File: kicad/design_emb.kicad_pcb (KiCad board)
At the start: 2 copper layers, 79.9 x 98.8 mm, 116 parts, among them J1 Conn_01x04, J2 Barrel_Jack, J3 USB_A, J4 Conn_01x03, J5 Conn_02x11_Counter_Clockwise, J6 Conn_02x10_Counter_Clockwise, J7 Screw_Terminal_01x02, J8 Screw_Terminal_01x02, K1 SANYOU_SRD_Form_C, K2 SANYOU_SRD_Form_C, Q1 MMBT3904, Q2 MMBT3904, SW1 SW_Push, SW3 SW_Push, U1 SRX.X.TCT, U10 S25FL116KOXNFIQ-11, U2 SRX.X.TCT, U3 STM32F446ZETx, U4 ICE40HX1K, U5 TLV1117LV33DCYR, U6 TLV1117LV33DCYR, U7 TLV1117LV12DCYR, U8 OMEGA2, U9 RCLAMP0502B

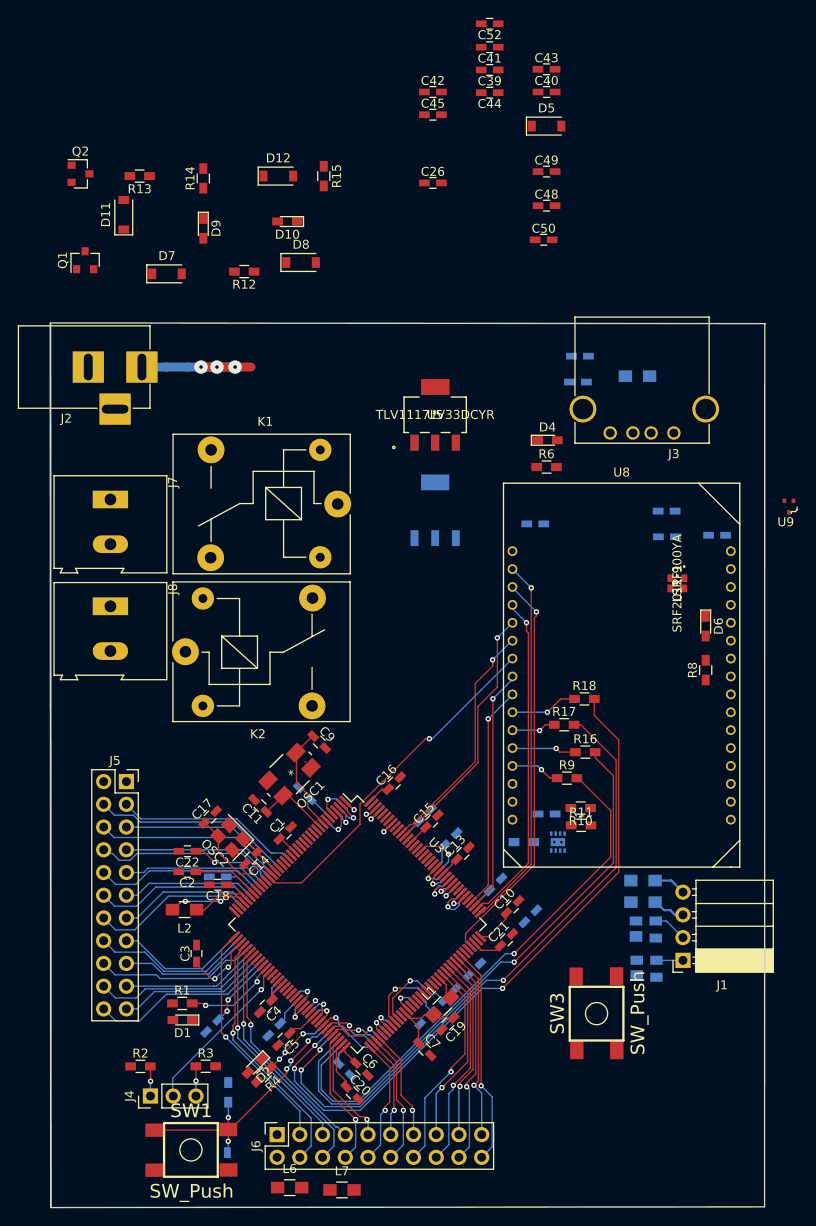
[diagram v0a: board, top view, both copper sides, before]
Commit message: ruteo
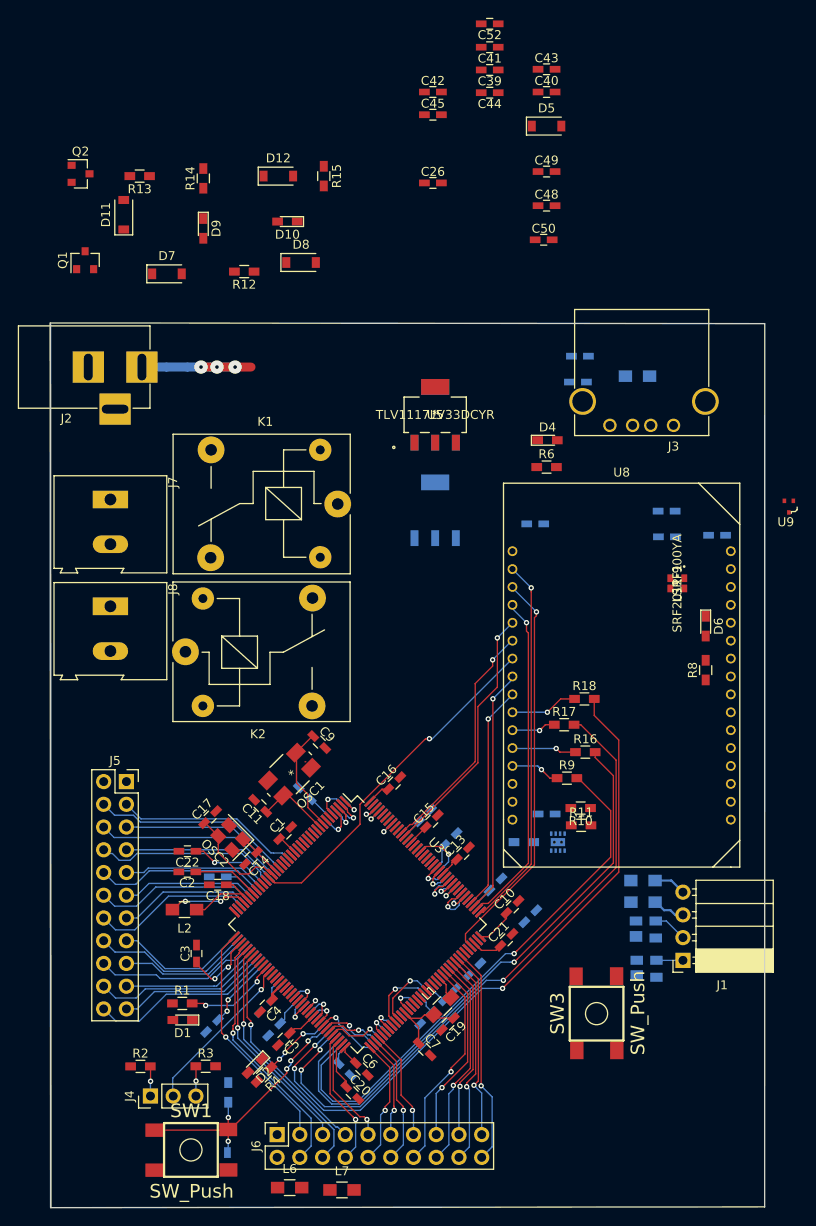
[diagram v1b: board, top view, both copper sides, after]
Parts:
- moved J3 0.85 mm to (148.8, 94.4)
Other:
- board size 79.9 x 98.8 mm -> 79.8 x 98.9 mm
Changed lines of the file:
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@@
   )
   (module Connectors:USB_A (layer F.Cu)
-    (at 148.844 95.25 180)
+    (at 148.8059 94.3991 180)
     (descr "USB A connector")
     (tags "USB USB_A")
@@
     )
   )
-  (gr_line (start 159.0802 83.0326) (end 79.1718 82.9564) (layer Edge.Cuts) (width 0.15))
-  (gr_line (start 158.9786 181.6989) (end 159.004 83.058) (layer Edge.Cuts) (width 0.15))
-  (gr_line (start 79.2353 181.7878) (end 79.1845 82.9818) (layer Edge.Cuts) (width 0.2))
+  (gr_line (start 158.9913 83.0326) (end 79.1718 82.9564) (layer Edge.Cuts) (width 0.15))
+  (gr_line (start 158.9913 181.7243) (end 159.004 83.058) (layer Edge.Cuts) (width 0.15))
+  (gr_line (start 79.2226 181.7878) (end 79.1718 82.9818) (layer Edge.Cuts) (width 0.2))
   (dimension 99.174366 (width 0.3) (layer F.SilkS)
-    (gr_text "99,174 mm" (at 73.454835 132.075698 89.93396571) (layer F.SilkS)
+    (gr_text "99,174 mm" (at 72.286058 132.546979 89.93396571) (layer F.SilkS)
       (effects (font (size 1.5 1.5) (thickness 0.3)))
     )
-    (feature1 (pts (xy 75.910241 82.491312) (xy 75.025564 82.490292)))
-    (feature2 (pts (xy 75.795941 181.665612) (xy 74.911264 181.664592)))
-    (crossbar (pts (xy 75.497684 181.665268) (xy 75.611984 82.490968)))
-    (arrow1a (pts (xy 75.611984 82.490968) (xy 76.197106 83.618147)))
-    (arrow1b (pts (xy 75.611984 82.490968) (xy 75.024265 83.616795)))
-    (arrow2a (pts (xy 75.497684 181.665268) (xy 76.085403 180.539441)))
-    (arrow2b (pts (xy 75.497684 181.665268) (xy 74.912562 180.538089)))
-  )
-  (gr_line (start 158.9532 181.7243) (end 79.2988 181.8005) (layer Edge.Cuts) (width 0.15))
+    (feature1 (pts (xy 74.741464 82.962593) (xy 73.856787 82.961573)))
+    (feature2 (pts (xy 74.627164 182.136893) (xy 73.742487 182.135873)))
+    (crossbar (pts (xy 74.328907 182.136549) (xy 74.443207 82.962249)))
+    (arrow1a (pts (xy 74.443207 82.962249) (xy 75.028329 84.089428)))
+    (arrow1b (pts (xy 74.443207 82.962249) (xy 73.855488 84.088076)))
+    (arrow2a (pts (xy 74.328907 182.136549) (xy 74.916626 181.010722)))
+    (arrow2b (pts (xy 74.328907 182.136549) (xy 73.743785 181.00937)))
+  )
+  (gr_line (start 158.9913 181.7243) (end 79.2099 181.8132) (layer Edge.Cuts) (width 0.15))
   (dimension 80.086204 (width 0.3) (layer F.SilkS)
     (gr_text "80,086 mm" (at 119.154383 183.078787 0.01817182924) (layer F.SilkS)
